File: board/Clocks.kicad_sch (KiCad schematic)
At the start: 21 parts, among them J10 Front Panel, J11 ATX-24, J5 0.89489MHz, J6 1.78977MHz, J7 3.57955MHz, J8 7.15909MHz, U39 74ACT14, U40 74F191, U43 DM1813-10, Y1 14.31818MHz

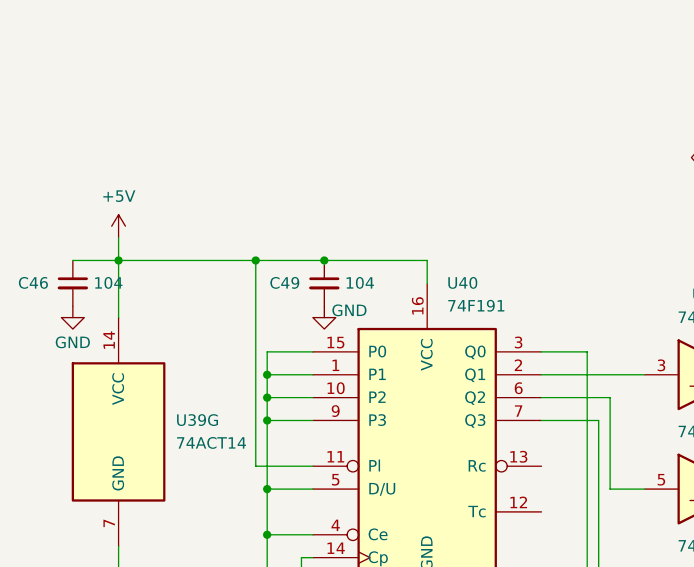
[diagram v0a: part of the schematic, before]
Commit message: bodge updates
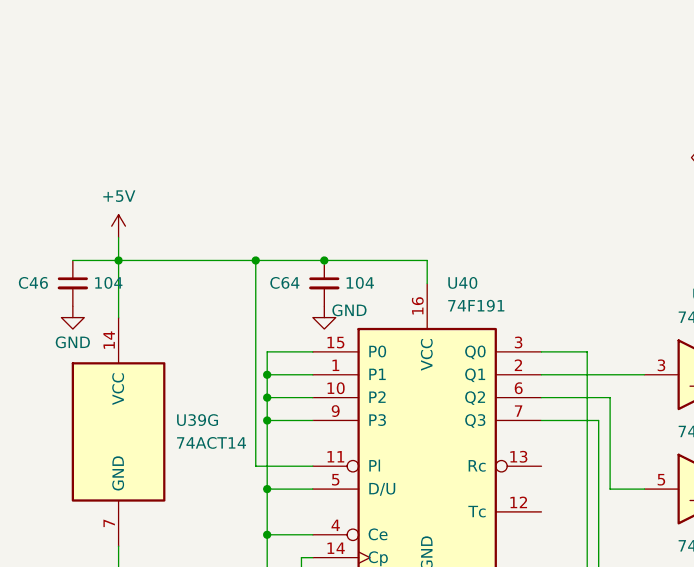
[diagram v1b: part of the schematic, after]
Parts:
- renumbered C49 to C64
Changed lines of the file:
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@@
 		(on_board yes)
 		(dnp no)
-		(property "Reference" "C49"
+		(property "Reference" "C64"
 			(at 62.484 73.66 0)
 			(effects
@@
 			(project "hydra-16"
 				(path "/ef29fc71-3fec-48b5-8a1a-46bee537a98c/9a593a77-f18f-43cb-9fdd-893618b7b90a"
-					(reference "C49")
+					(reference "C64")
 					(unit 1)
 				)
